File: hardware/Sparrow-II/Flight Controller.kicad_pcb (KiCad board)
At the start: 4 copper layers, 41 x 41 mm, 103 parts

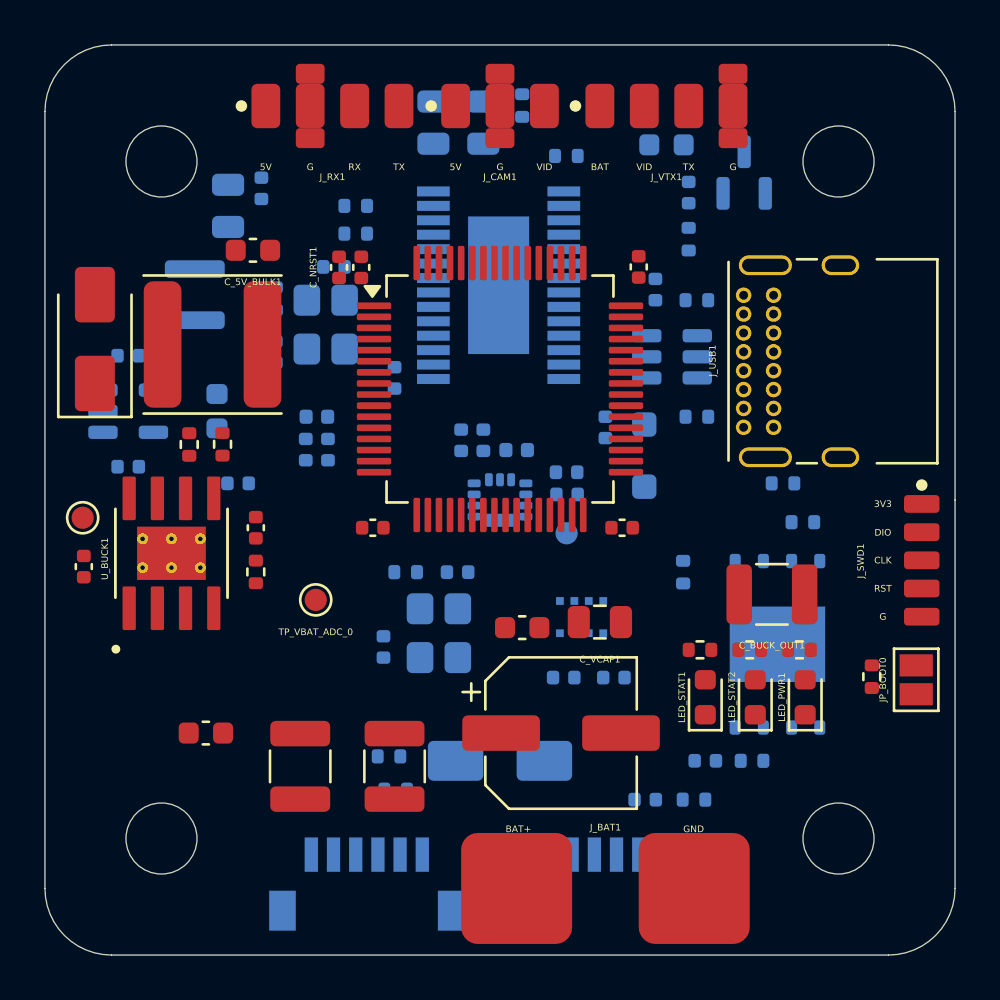
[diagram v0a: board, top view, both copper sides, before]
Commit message: hardware: layout checkpoint 1
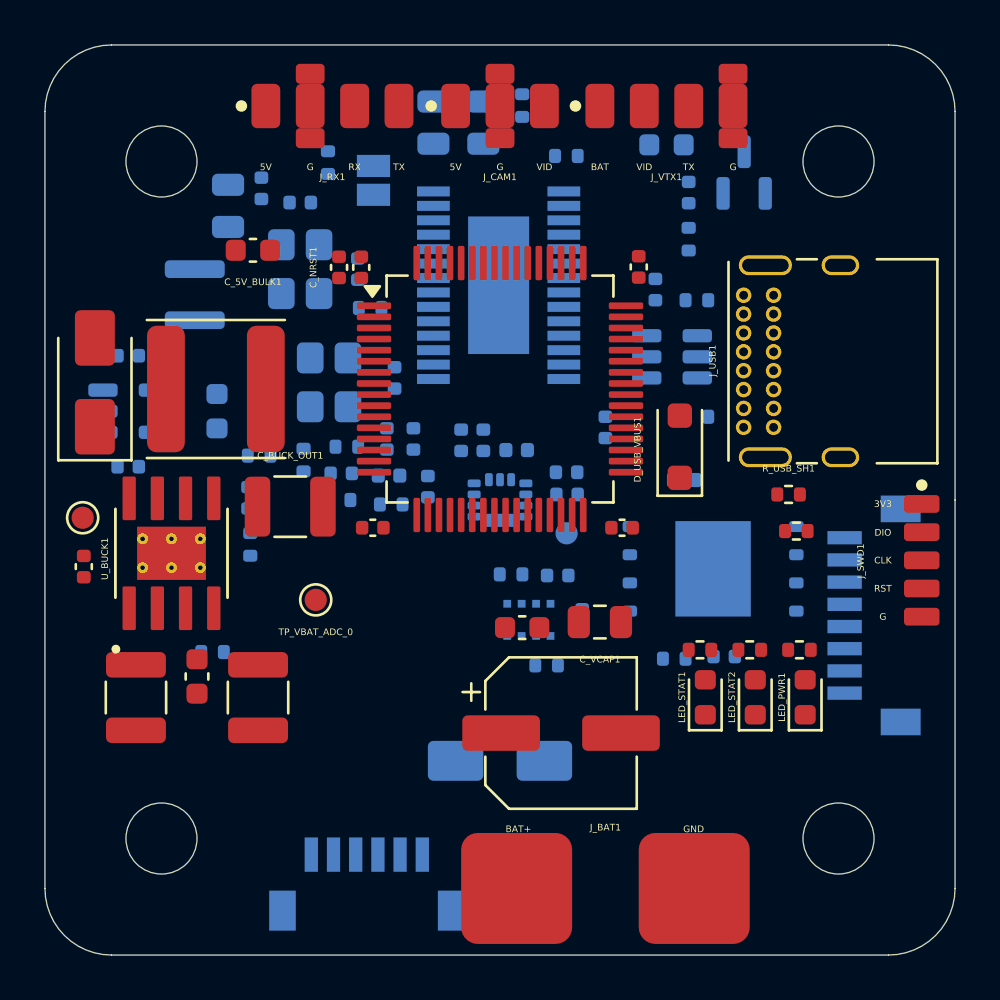
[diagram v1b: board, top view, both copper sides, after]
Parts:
- C_BUCK_SS1, JP_BOOT0, R_BOOT0, R_BUCK_FB1, R_BUCK_FB2, R_BUCK_RT1: moved to B.Cu
- D_USB_VBUS1, R_FLASH_CS1, R_USB_SH1: moved to F.Cu
- moved R_BOOT0 33.7 mm to (142.2, 84.8)
- moved JP_BOOT0 33.2 mm to (144.3, 85.6)
- moved R_CURR_F1 23.3 mm to (141.2, 98.2), turned to 90 degrees
- moved R_I2C_SCL1 22.4 mm to (152.1, 107.5)
- moved C_BUCK_OUT1 22.1 mm to (140.6, 100.3), turned to 0 degrees
- moved C_CURR_F1 20.1 mm to (142.8, 98.8), turned to 0 degrees
- moved J_ESC1 17.1 mm to (167.3, 105.2), turned to 90 degrees
- moved R_I2C_SDA1 16.9 mm to (150.5, 103.3), turned to 0 degrees
- moved C_HSE1 12.9 mm to (139.8, 93.3), turned to 90 degrees
- moved R_VBAT_D2 12.9 mm to (145.1, 100.2)
- moved Y_HSE1 12.3 mm to (142.3, 94.7), turned to 90 degrees
- moved C_HSE2 12.2 mm to (139.8, 95.5), turned to 90 degrees
- moved R_VBAT_D1 11.8 mm to (142.8, 100.0)
- moved C_VBAT_ADC1 8.55 mm to (146.8, 99.4), turned to 90 degrees
- moved C_BUCK_IN1 8.02 mm to (133.6, 108.9)
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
